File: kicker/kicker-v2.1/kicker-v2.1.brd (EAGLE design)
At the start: 140 x 149.9 mm, 86 parts, among them IC1 MEGA8-AI, J1 1X2-3.5MM, J2 1X2-3.5MM, J3 XT-60BATT_LABEL, J4 1X2-3.5MM, J5 1X2-3.5MM, J6 1X2-3.5MM, J7 1X2-3.5MM, Q3 16MHz, T1 BC547, T2 BC547

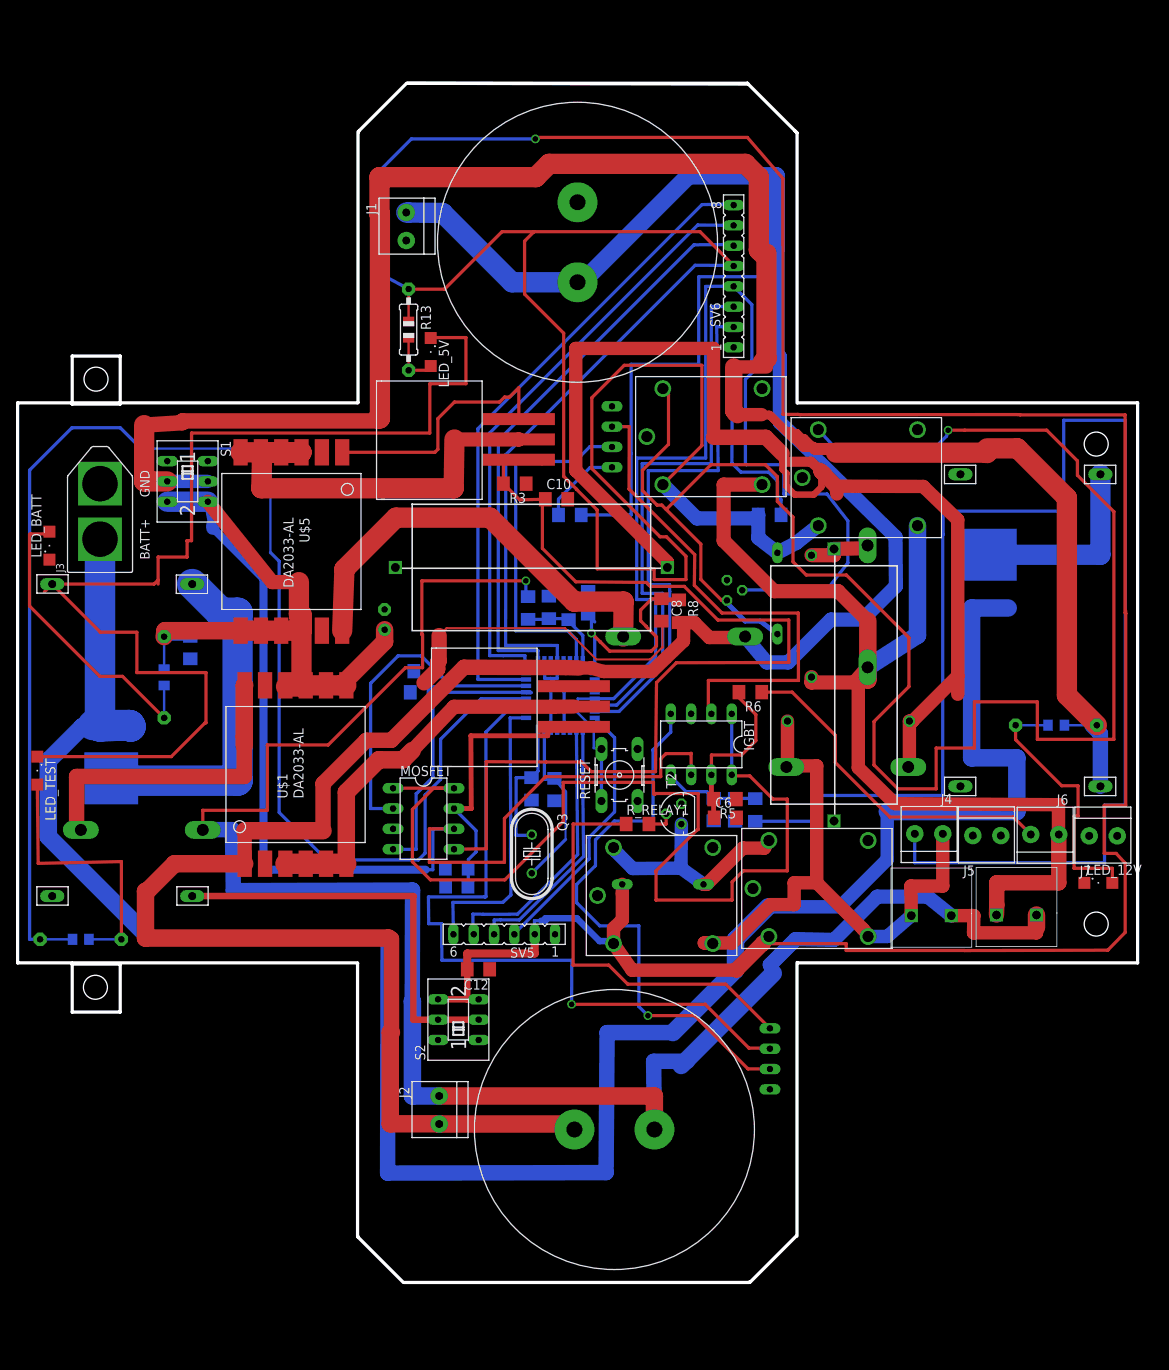
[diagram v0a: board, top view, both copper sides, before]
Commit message: Kicker proto
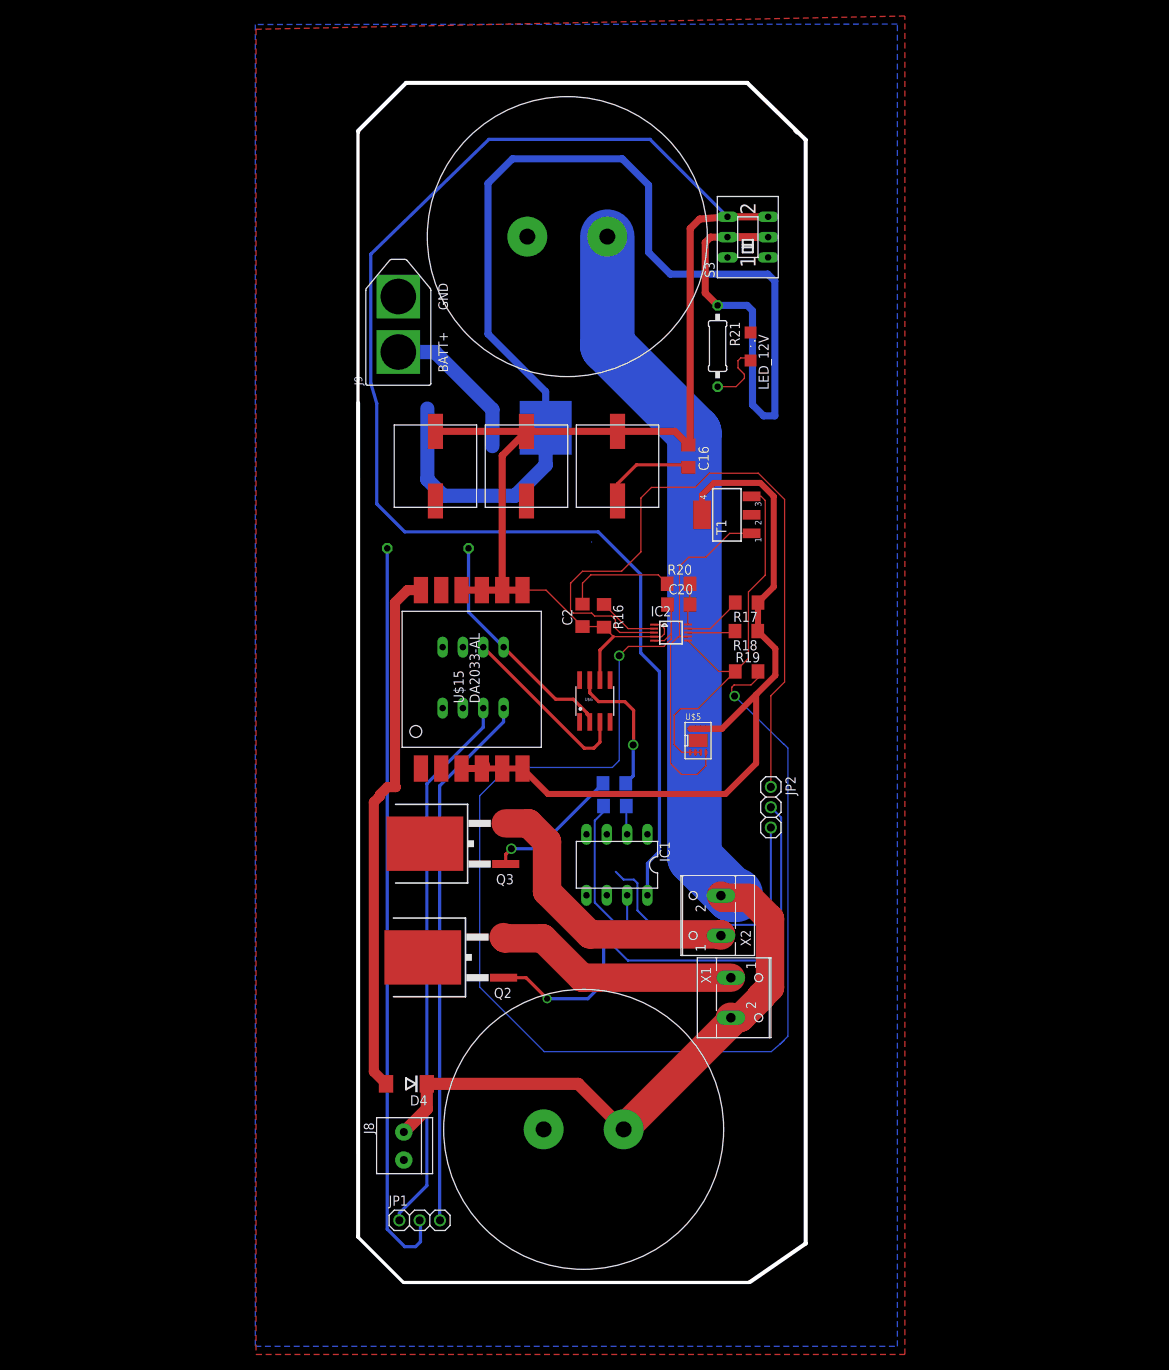
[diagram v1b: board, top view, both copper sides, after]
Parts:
- removed !RESET: (no value), switch-omron:B3F-10XX
- removed 5V, GND, GND12, GND_12V1, GND_5V, POWER_1, POWER_HEAD1, V_BAT: PINHEAD_1, pinhead_1:PINHEAD_1
- removed C1, C10, C11, C6, C8, C9: 0.01uF, rcl:C1206
- removed C12: 0.1uF, rcl:C1206
- removed C13, C14: 22pF, rcl:C1206
- removed C3: 4.7uF, rcl:C1206
- removed C4: 4.7uF, rcl:E2,5-6
- removed D1, D2, DS, DS1: UF5400, diode-1:DO201-15
- removed D3, D5: 1N4446, diode:DO35-10
- removed FHEADER1, FHEADER4: F-1X04-SIP-100-32Y, con-headers-jp:SIP-100-04-32Y
- removed IGBT, MOSFET: NE555, st-microelectronics:DIL-08
- removed J1, J2, J4, J5, J6, J7: 1X2-3.5MM, adafruit:1X2-3.5MM
- removed J3: XT-60BATT_LABEL, RoboJackets-Connectors:XT-60
- removed LED_5V, LED_BATT, LED_TEST: (no value), led:SML1206
- removed R10, R12, R4: 10K, resistor:R1206
- removed R11, R6: 330, resistor:R1206
- removed R13, R9: 1 K, adafruit:0805-THM
- removed R14, R15: 4.7 K, adafruit:0805-THM
- removed R7, RD2: 8.2K, resistor:R1206
- removed R8, RD1: 1M, resistor:R1206
- removed RS, RS1: 10/.5W, rcl:0411/15
- removed R_RELAY, R_RELAY1: 1K, resistor:R1206
- removed S1, S2: (no value), switch:A68-A31
- removed SV5: (no value), con-lsta:FE06
- removed SV6: (no value), con-lsta:FE08
- removed T2: BC547, transistor:TO92
- removed U$10, U$11, U$12, U$13: REL, rel:REL
- removed U$16: SCREW, screw:SCREW
- removed U$7, U$8: POLYCAP, polycap:POLYCAP
- removed U$9: MOS, mosfet:MOS
- removed U4: (no value), LP38690DT-3.3:TO228P1042X238-3N
- added C16, C2, C20: (no value), rcl:C1206
- added D4: (no value), diode:DO214AA
- added IC2: AD7992, analog_devices_gaui:MSOP10
- added IC4: NE555, st-microelectronics:DIL-08
- added J8: 1X2-3.5MM, adafruit:1X2-3.5MM
- added J9: XT-60BATT_LABEL, RoboJackets-Connectors:XT-60
- added JP1, JP2: (no value), adafruit:1X03
- added Q2: SPB80P06P, transistor-fet:TO263
- added R16, R17, R18, R20: (no value), adafruit:R1206
- added R19: (no value), resistor:R1206
- added R21: 4.7 K, resistor:0207/10
- added S3: (no value), switch:A68-A31
- added U$15: DA2033-AL, inductor-coilcraft-2:DA2033-AL
- added U$17: (no value), Electrolytic-Cap:CAP
- added X1, X2: (no value), con-wago-500:W237-102
- IC1: value MEGA8-AI -> NE555; device atmel:TQFP32-08 -> st-microelectronics:DIL-08
- Q3: value 16MHz -> SPB80P06P; device crystal:HC49U70 -> transistor-fet:TO263
- R1, R3: value 1K -> (none); device resistor:R1206 -> adafruit:R1206
- R2: value 10K -> (none); device resistor:R1206 -> adafruit:R1206
- R5: value 10K -> 4.7 K; device resistor:R1206 -> resistor:0207/10
- T1: value BC547 -> (none); device transistor:TO92 -> transistor-neu-to92:SOT223
- U$1: value DA2033-AL -> CAP; device inductor-coilcraft-2:DA2033-AL -> SVP_F12:SVP_F12
- U$3: value MOS -> CAP; device mosfet:MOS -> SVP_F12:SVP_F12
- U$4: value (none) -> CAP; device Electrolytic-Cap:CAP -> SVP_F12:SVP_F12
- U$5: value DA2033-AL -> MOSFET-LT3750; device inductor-coilcraft-2:DA2033-AL -> SON-8:SON-8
- U$6: value SCREW -> TC4426A; device screw:SCREW -> smd-footprints:SOIC-8
- moved LED_12V 79.9 mm to (91.8, 77.2), turned to 270 degrees
- moved U1 57.9 mm to (66.0, 67.0), turned to 90 degrees
- moved U$5 56.6 mm to (85.2, 27.9), turned to 0 degrees
- moved U$1 56.0 mm to (70.0, 67.4), turned to 0 degrees
- moved U$6 49.9 mm to (72.3, 32.9), turned to 0 degrees
- moved R5 48.6 mm to (51.5, 52.0), flipped to the bottom
- moved R3 39.5 mm to (74.8, 22.6), flipped to the bottom, turned to 0 degrees
- moved U$3 36.7 mm to (58.6, 67.4)
- moved U$4 32.3 mm to (47.3, 67.4), turned to 0 degrees
- moved R2 29.1 mm to (74.8, 19.8), turned to 0 degrees
- moved IC1 22.3 mm to (75.1, 12.4), flipped to the top, turned to 180 degrees
- moved R1 21.4 mm to (74.8, 3.65), turned to 0 degrees
- moved Q3 9.94 mm to (54.6, 15.0), turned to 90 degrees
- moved T1 9.43 mm to (88.8, 56.2), flipped to the top
- moved U$2 3.85 mm to (70.9, -20.7)
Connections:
- removed net !RESET: !RESET.1, !RESET.2, IC1.29, R12.1, SV6.4
- removed net ATMEGA_POW: C12.2, D3.C, D5.C, IC1.18, IC1.20, IC1.4, IC1.6, R12.2, R13.1, S2.3, S2.6, SV5.2, SV6.5, U$10.2, U$11.2, U$12.2, U$13.2
- removed net ATMEGA_POW_BS: 5V.P$1, S2.2, S2.5
- removed net BATT: C3.1, C4.+, IGBT.6, MOSFET.6, R14.1, S1.3, S1.6, U$1.P$10, U$1.P$7, U$1.P$8, U$1.P$9, U$5.P$10, U$5.P$7, U$5.P$8, U$5.P$9
- removed net C1+: D1.C, J2.1, RD1.2, U$16.+, U$2.P$2, U$6.+
- removed net C1-: D2.C, J1.1, J2.2, R8.2, U$1.P$1, U$2.P$1, U$4.P$2
- removed net COLLECTOR: D3.A, T1.3, U$10.1, U$12.1
- removed net COLLECTOR1: D5.A, T2.3, U$11.1, U$13.1
- removed net DRV_IN: J6.2, R6.1
- removed net DRV_IN1: J4.2, R11.1
- removed net EXT1: IC1.32, SV5.3
- removed net EXT2: IC1.1, SV5.4
- removed net FEED1: C9.1, IC1.24, RD1.1, RD2.2
- removed net FEED2: C8.1, IC1.25, R7.2, R8.1
- removed net GND1: GND.P$1, LED_5V.C, LED_TEST.C
- removed net GPIO: IC1.2, SV5.5
- removed net GPIO1: IC1.9, SV5.6
- removed net IGBT1: FHEADER1.2, IGBT.2
- removed net IGBT2: FHEADER4.2, IGBT.4
- removed net MISO16: IC1.16, SV6.7
- removed net MOS1: IC1.14, MOSFET.2, R2.2
- removed net MOS2: IC1.13, MOSFET.4, R4.2
- removed net MOSI15: IC1.15, SV6.8
- removed net N$11: R_RELAY1.2, T2.2
- removed net N$12: LED_BATT.A, R14.2
- removed net N$14: C13.2, IC1.7, Q3.2
- removed net N$15: LED_12V.A, R15.2
- removed net N$16: U4.2, V_BAT.P$1
- removed net N$17: C14.2, IC1.8, Q3.1
- removed net N$19: LED_TEST.A, R9.2
- removed net N$21: U$5.P$3, U$5.P$4, U$5.P$5, U$5.P$6, U$9.DRAIN
- removed net N$22: U$1.P$3, U$1.P$4, U$1.P$5, U$1.P$6, U$3.DRAIN
- removed net N$23: IC1.12, R9.1
- removed net N$6: LED_5V.A, R13.2
- removed net N$7: POWER_HEAD1.P$1, U1.2
- removed net N$8: D1.A, U$1.P$12
- removed net N$9: DS1.C, RS1.1, U$8.1
- removed net NC: IGBT.1, IGBT.8, MOSFET.1, MOSFET.8
- removed net OUTB: C1.1, IGBT.5, R10.2, R11.2
- removed net POWER: POWER_1.P$1, R15.1, S1.2, S1.5
- removed net PWM1: C11.1, MOSFET.7, R1.2, U$3.GATE
- removed net PWM2: C10.1, MOSFET.5, R3.2, U$9.GATE
- removed net RELAY: FHEADER1.4, R_RELAY.1
- removed net RELAY1: FHEADER4.4, R_RELAY1.1
- removed net RXD30: IC1.30, SV6.3
- removed net S+: DS.A, J6.1, RS.2, U$10.NO, U$12.NO, U$16.-
- removed net S1+: DS1.A, J4.1, RS1.2, U$11.NO, U$13.NO, U$6.-
- removed net SCK17: IC1.17, SV6.6
- removed net SWITCH: FHEADER1.3, IC1.23
- removed net SWITCH1: FHEADER4.3, IC1.10
- removed net TXD31: IC1.31, SV6.2
- new net 3.3V: IC4.1, JP1.3
- new net 5.0V: JP1.2, R5.1
- new net ANODE(+)_1: IC1.2, R2.1
- new net C+: D4.C, J8.1, U$17.P$2, U$2.P$2, X1.2, X2.2
- new net CHARGE: IC2.3, JP2.1
- new net DONE: IC2.2, R16.1
- new net GATE: IC2.7, T1.1, U$5.4
- new net GATE_IGBT_1: Q2.1, R1.2
- new net GATE_IGBT_2: Q3.1, R3.2
- new net MOS_TRIG: IC4.2, JP1.1
- new net N$28: D4.A, U$15.P$12
- new net N$29: LED_12V.A, R21.2
- new net PIN3: IC4.7, U$6.3
- new net RDCM: IC2.8, R18.2
- new net RGB: C20.2, IC2.10, R20.2
- new net RVOUT: IC2.9, R17.2
- new net SOURCE: IC2.6, R19.1, T1.3, U$5.1, U$5.2, U$5.3
- new net SUPP_+: R21.1, S3.2, S3.5, U1.2
- new net TRIG_ON_1: JP2.2, R2.2
- new net TRIG_ON_2: JP2.3
- new net VO/NC_1: IC1.6
- new net VO_1: IC1.7, R1.1
- new net VO_2: R3.1, U$6.7
- new net VTRANS: C16.1, C2.1, IC1.8, IC2.1, IC2.4, R16.2, S3.3, S3.6, U$1.+, U$15.P$10, U$15.P$7, U$15.P$8, U$15.P$9, U$3.+, U$4.+, U$6.6
- net GND: now also C16.2, C2.2, C20.1, IC1.1, IC2.5, J8.2, J9.GND, Q2.3, Q3.3, R19.2, R20.1, U$1.-, U$15.P$1, U$17.P$1, U$2.P$1, U$3.-, U$4.-; no longer !RESET.3, !RESET.4, C1.2, C10.2, C11.2, C12.1, C13.1, C14.1, C3.2, C4.-, C6.2, C8.2, C9.2, FHEADER1.1, FHEADER4.1, GND12.P$1, GND_12V1.P$1, GND_5V.P$1, IC1.21, IGBT.3, J1.2, J3.GND, J5.1, J7.1, LED_BATT.C, MOSFET.3, R1.1, R10.1, R2.1, R3.1, R4.1, R5.1, R7.1, RD2.1, SV5.1, SV6.1, T1.1, T2.1, U$10.C, U$11.C, U$12.C, U$13.C, U$3.SOURCE, U$4.P$1, U$5.P$1, U$7.2, U$8.2, U$9.SOURCE
- net N$1: now also Q2.2, X1.1; no longer DS.C, RS.1, U$7.1
- net N$2: now also Q3.2, X2.1; no longer R_RELAY.2, T1.2
- net N$3: now also R17.1, R18.1, T1.4, U$15.P$3, U$15.P$4, U$15.P$5, U$15.P$6, U$5.5, U$5.6, U$5.7, U$5.8; no longer C6.1, IGBT.7, R5.2, R6.2
- net N$4: now also IC4.8, R5.2, U$6.2; no longer D2.A, U$5.P$12
- net POWER_HEAD: now also J9.BATT; no longer J3.BATT, U4.1, U4.3
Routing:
- net ATMEGA_POW: track 613.7 -> 0.00 mm, vias 1 -> 0
- net C1-: track 319.5 -> 0.00 mm
- net VTRANS: track 0.00 -> 291.3 mm
- net POWER: track 283.4 -> 0.00 mm
- net POWER_HEAD: track 280.0 -> 19.3 mm
- net C1+: track 259.4 -> 0.00 mm, vias 1 -> 0
- net COLLECTOR: track 226.5 -> 0.00 mm, vias 1 -> 0
- net BATT: track 207.6 -> 0.00 mm
- net N$23: track 189.6 -> 0.00 mm
- net DRV_IN1: track 181.6 -> 0.00 mm
- net SUPP_+: track 0.00 -> 171.0 mm
- net C+: track 0.00 -> 167.2 mm
- net N$9: track 146.2 -> 0.00 mm
- net GND1: track 144.5 -> 0.00 mm
- net S+: track 131.9 -> 0.00 mm
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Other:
- board size 140 x 149.9 mm -> 56 x 149.9 mm
